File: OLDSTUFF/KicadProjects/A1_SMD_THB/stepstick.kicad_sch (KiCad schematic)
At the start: 22 parts, among them M101 StepperMotor, U104 TMC2209-LA

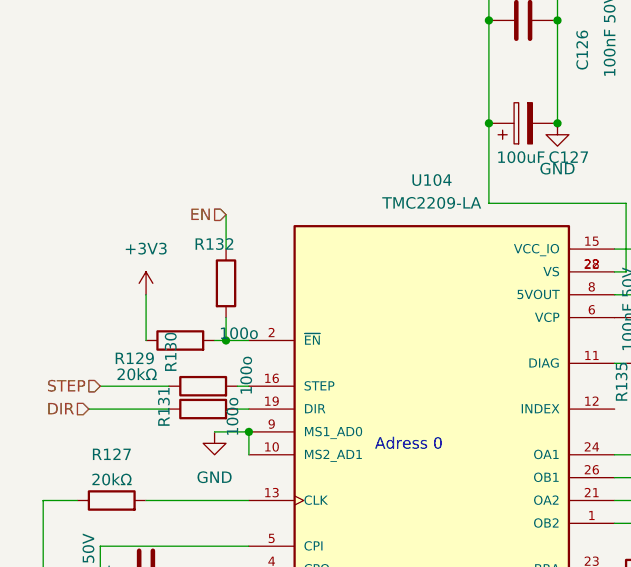
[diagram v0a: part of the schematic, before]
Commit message: e
e
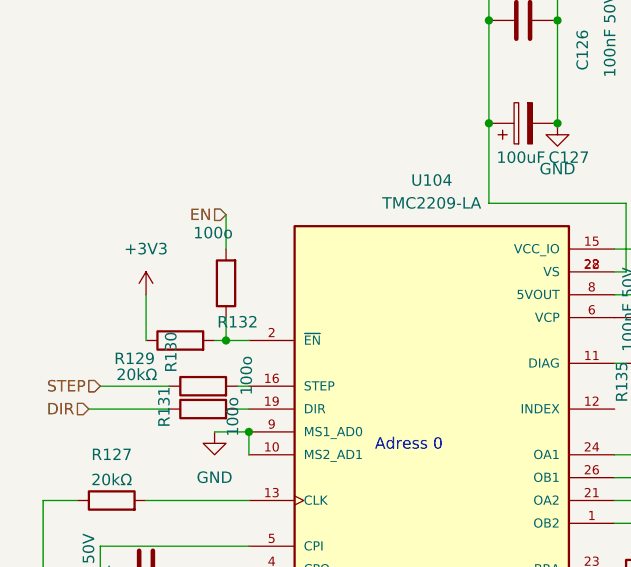
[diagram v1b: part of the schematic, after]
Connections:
- net EN: now also R132.2; no longer R132.1
- net at R129.2, U104.2 (~{EN}): now also R132.1; no longer R132.2
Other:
- moved on the sheet: R132
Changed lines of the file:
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@@
 	(symbol
 		(lib_id "Device:R")
-		(at 39.37 58.42 0)
+		(at 39.37 58.42 180)
 		(unit 1)
 		(exclude_from_sim no)
@@
 		(dnp no)
 		(property "Reference" "R132"
-			(at 35.814 54.102 0)
+			(at 42.926 62.738 0)
 			(effects
 				(font
@@
 		)
 		(property "Value" "100o"
-			(at 38.608 64.008 0)
+			(at 40.132 52.832 0)
 			(effects
 				(font
@@
 		)
 		(property "Footprint" "Resistor_SMD:R_0402_1005Metric"
-			(at 37.592 58.42 90)
+			(at 41.148 58.42 90)
 			(effects
 				(font
